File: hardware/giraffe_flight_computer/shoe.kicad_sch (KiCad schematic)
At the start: 70 parts, among them J8 USB, J9 EXT_AUDIO, K1 TLP241A, U10 PCM2902C, U11 TLP185, U12 ISO6720B, U13 74LVC1G04, U6 TLP185, Y1 12MHz

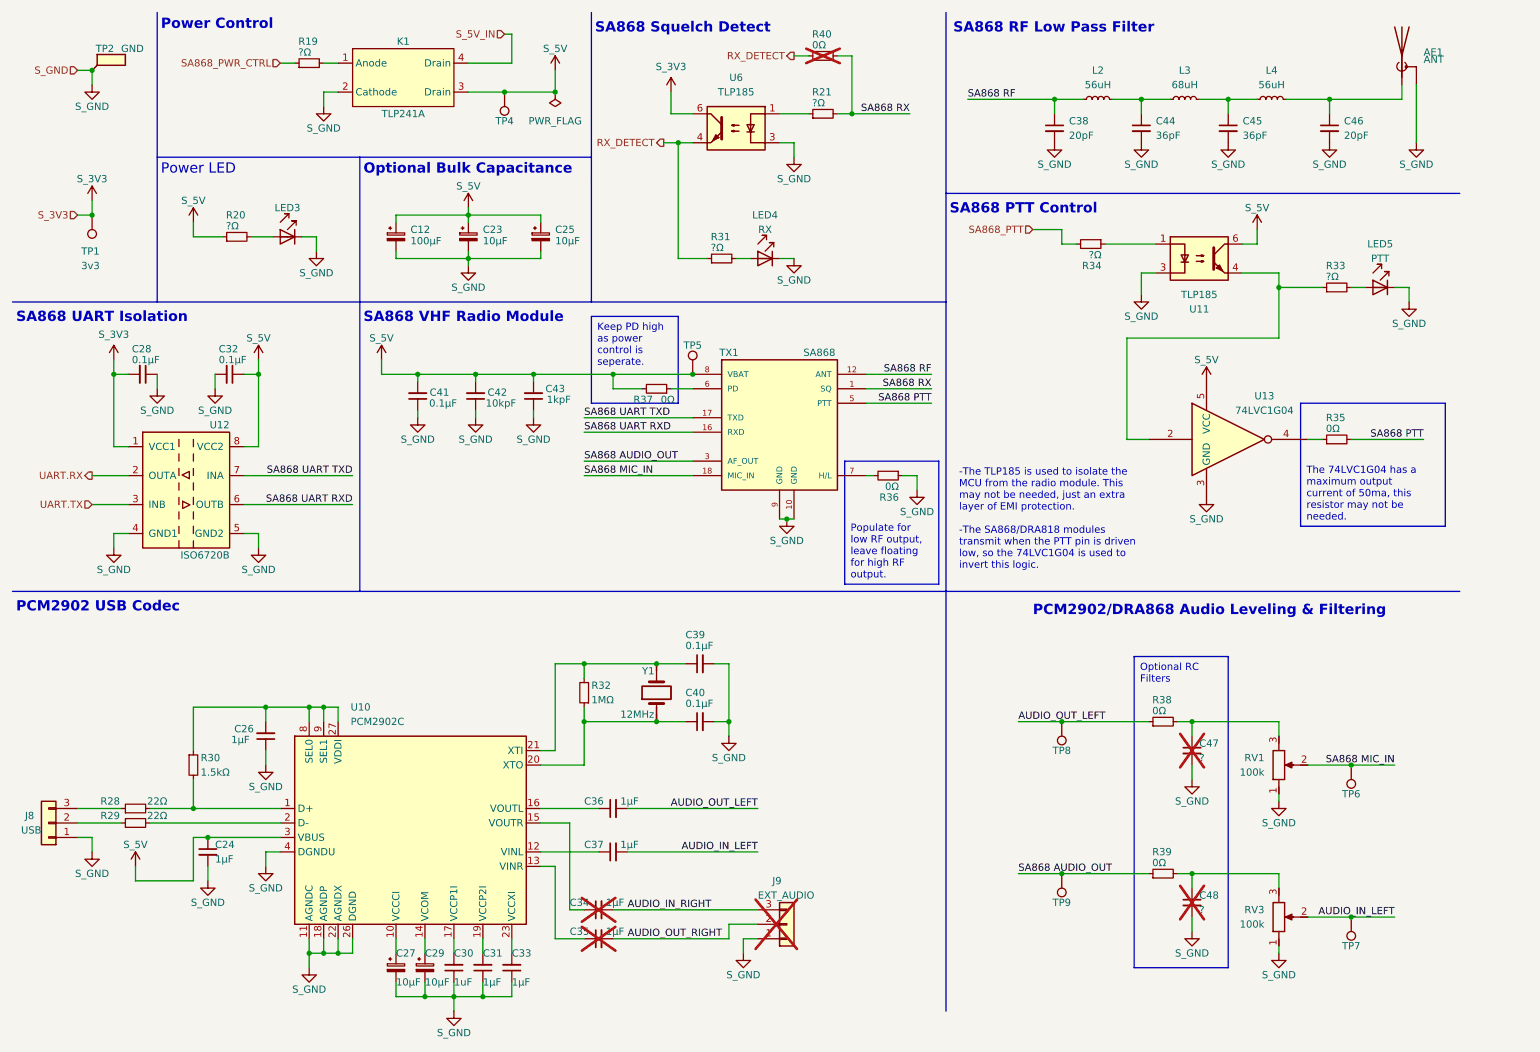
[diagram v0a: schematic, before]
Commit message: reorganization
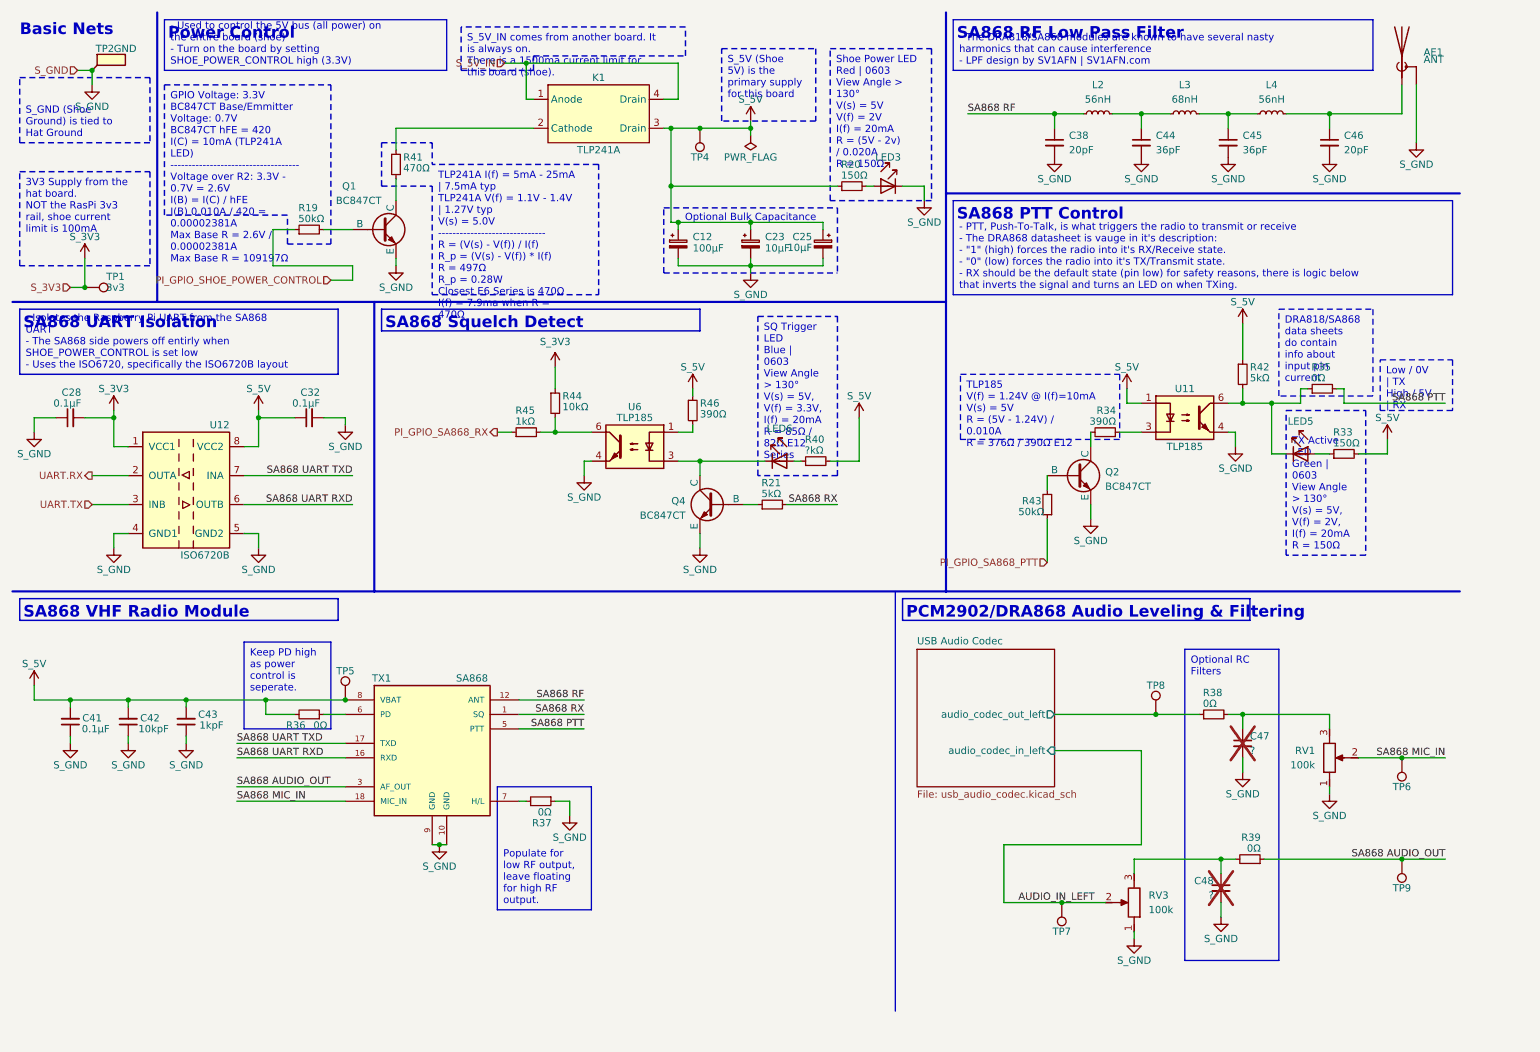
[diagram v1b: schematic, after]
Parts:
- removed C24, C31, C33, C34, C35, C36, C37: 1μF, Resistor_SMD:R_0805_2012Metric, symbol Device:C_Small
- removed C26: 1μF, Capacitor_SMD:C_0603_1608Metric, symbol Device:C_Small
- removed C27, C29: 10μF, Resistor_SMD:R_1210_3225Metric, symbol Device:C_Polarized_Small
- removed C30: 1uF, Resistor_SMD:R_0805_2012Metric, symbol Device:C_Small
- removed C39, C40: 0.1μF, Resistor_SMD:R_0805_2012Metric, symbol Device:C_Small
- removed J8: USB, Connector_PinHeader_1.00mm:PinHeader_1x03_P1.00mm_Vertical, symbol Connector_Generic:Conn_01x03
- removed J9: EXT_AUDIO, Connector_PinHeader_1.00mm:PinHeader_1x03_P1.00mm_Vertical, symbol Connector_Generic:Conn_01x03
- removed LED4: RX, LED_SMD:LED_0603_1608Metric, symbol giraffe_symbols:Generic_LED
- removed R28, R29: 22Ω, Resistor_SMD:R_0603_1608Metric, symbol Device:R_Small
- removed R30: 1.5kΩ, Resistor_SMD:R_0603_1608Metric, symbol Device:R_Small
- removed R31: ?Ω, Resistor_SMD:R_0603_1608Metric, symbol Device:R_Small
- removed R32: 1MΩ, Resistor_SMD:R_0603_1608Metric, symbol Device:R_Small
- removed U10: PCM2902C, Package_SO:SSOP-28_5.3x10.2mm_P0.65mm, symbol giraffe_symbols:PCM2902
- removed U13: 74LVC1G04, Package_TO_SOT_SMD:SOT-353_SC-70-5, symbol giraffe_symbols:74LVC1G04
- removed Y1: 12MHz, Crystal:Crystal_SMD_0603-2Pin_6.0x3.5mm, symbol giraffe_symbols:Crystal
- added LED6: ~, LED_SMD:LED_0603_1608Metric, symbol giraffe_symbols:Generic_LED
- added Q1, Q2, Q4: BC847CT, symbol Simulation_SPICE:NPN
- added R41: 470Ω, Resistor_SMD:R_0603_1608Metric, symbol Device:R_Small
- added R42: 5kΩ, Resistor_SMD:R_0603_1608Metric, symbol Device:R_Small
- added R43: 50kΩ, Resistor_SMD:R_0603_1608Metric, symbol Device:R_Small
- added R44: 10kΩ, Resistor_SMD:R_0603_1608Metric, symbol Device:R_Small
- added R45: 1kΩ, Resistor_SMD:R_0603_1608Metric, symbol Device:R_Small
- added R46: 390Ω, Resistor_SMD:R_0603_1608Metric, symbol Device:R_Small
- L2, L4: value 56uH -> 56nH
- L3: value 68uH -> 68nH
- LED5: value PTT -> ~
- R19: value ?Ω -> 50kΩ
- R20, R33: value ?Ω -> 150Ω
- R21: value ?Ω -> 5kΩ
- R34: value ?Ω -> 390Ω
- R40: value 0Ω -> ?kΩ; now fitted
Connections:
- net SA868 RX: no longer R40.2
- net S_3V3: now also R44.1; no longer U6.6
- net S_5V: now also R33.2, R36.2, R40.2, U11.1, R42.1, R46.1; no longer R37.2, U11.6
- net S_5V_IN: now also K1.1 (Anode)
- net S_GND: now also R37.1, U11.4, U6.4, Q1.3 (E), Q2.3 (E), Q4.3 (E); no longer K1.2 (Cathode), LED5.1 (K), R36.1, U11.3, U6.3
- net at R35.1: now also LED5.1 (K), U11.6, R42.2
- net at R21.1: now also Q4.2 (B); no longer U6.1
- net at TX1.6 (PD): now also R36.1; no longer R37.1
- net at LED5.2 (A): now also R33.1; no longer R33.2
- net at TX1.7 (H/L): now also R37.2; no longer R36.2
- net at R19.2: now also Q1.2 (B); no longer K1.1 (Anode)
- net at R34.1: now also U11.3; no longer U11.1
- net AUDIO_OUT_LEFT renamed USB Audio Codec/audio_codec_out_left
- net RX_DETECT: no longer names the net of R40.1
- net RX_DETECT: now also LED6.2 (A); no longer U6.4
- net SA868_PTT: no longer names the net of R34.2
- net SA868_PTT: now also Q2.1 (C)
- net SA868_PWR_CTRL renamed PI_GPIO_SHOE_POWER_CONTROL
- new net: R44.2, R45.2, U6.6
- new net: LED6.1 (K), Q4.1 (C), U6.3
- new net: Q2.2 (B), R43.2
- new net: Q1.1 (C), R41.2
- new net: K1.2 (Cathode), R41.1
- new net: R46.2, U6.1
- new net PI_GPIO_SA868_PTT: R43.1
- new net PI_GPIO_SA868_RX: R45.1
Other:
- added sheet USB Audio Codec (usb_audio_codec.kicad_sch)
- note added: "Basic Nets"
- note removed: "PCM2902 USB Codec"
- note removed: "Power LED"
- moved on the sheet: C38, C44, C45, C46, C47, C48, K1, L2, L3, L4, R38, R39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
